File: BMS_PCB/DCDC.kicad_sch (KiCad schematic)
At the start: 26 parts, among them IC1 TPS560430XFDBVT, U4 TPS70933DBVT

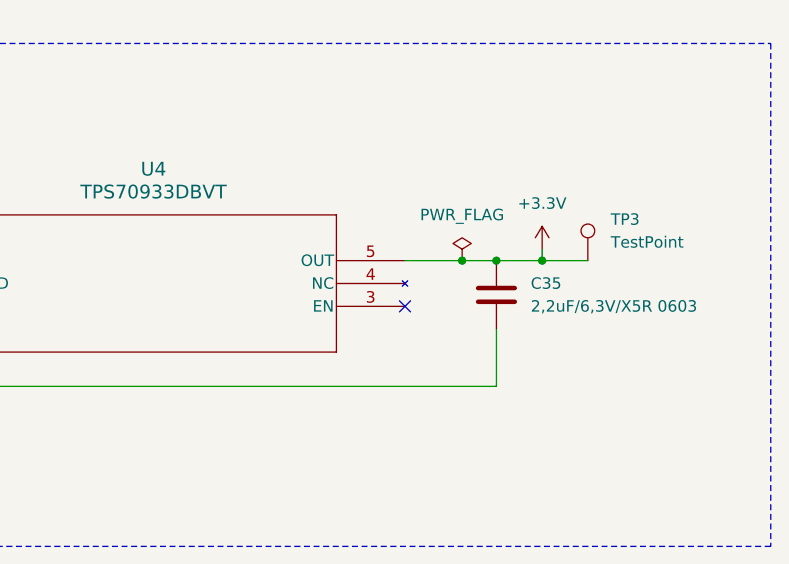
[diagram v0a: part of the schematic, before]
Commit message: Sonntag, 04.05.
Leiterbahndicken angepasst, Bohrlöcher erneuert, µC final angeschlossen, letzte Bugfixes
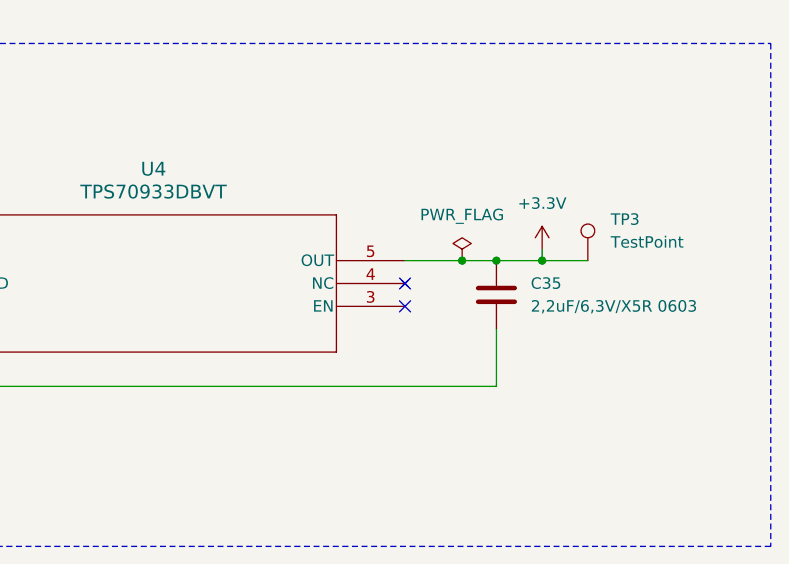
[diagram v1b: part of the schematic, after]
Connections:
- no-connect marks 3 -> 4
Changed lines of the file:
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@@
 		(at 78.74 53.34)
+	)
+	(no_connect
+		(at 233.68 116.84)
 	)
 	(wire

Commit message: Bugfix
Capacity und Resistors
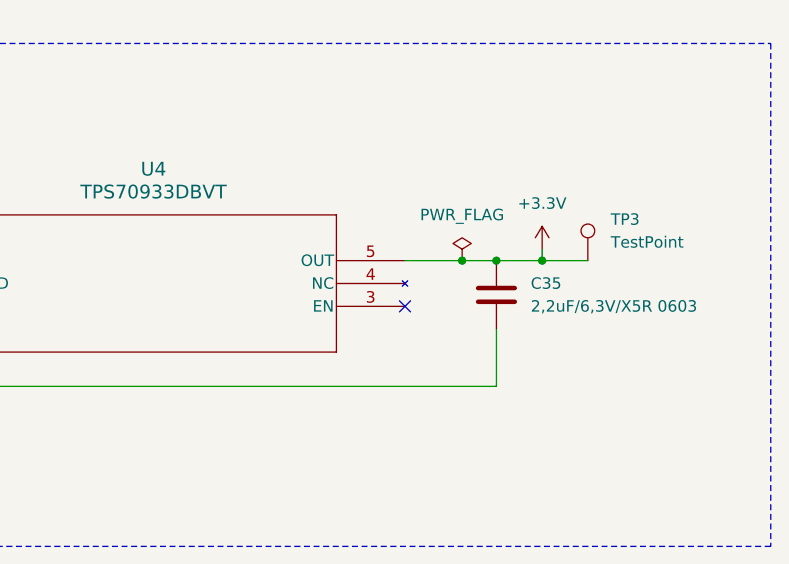
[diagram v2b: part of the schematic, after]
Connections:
- no-connect marks 4 -> 3
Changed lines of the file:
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@@
 		(at 78.74 53.34)
-	)
-	(no_connect
-		(at 233.68 116.84)
 	)
 	(wire
